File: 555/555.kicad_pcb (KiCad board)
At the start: 2 copper layers, 10 parts, among them U1 LM555xM, U2 TSOP17xx

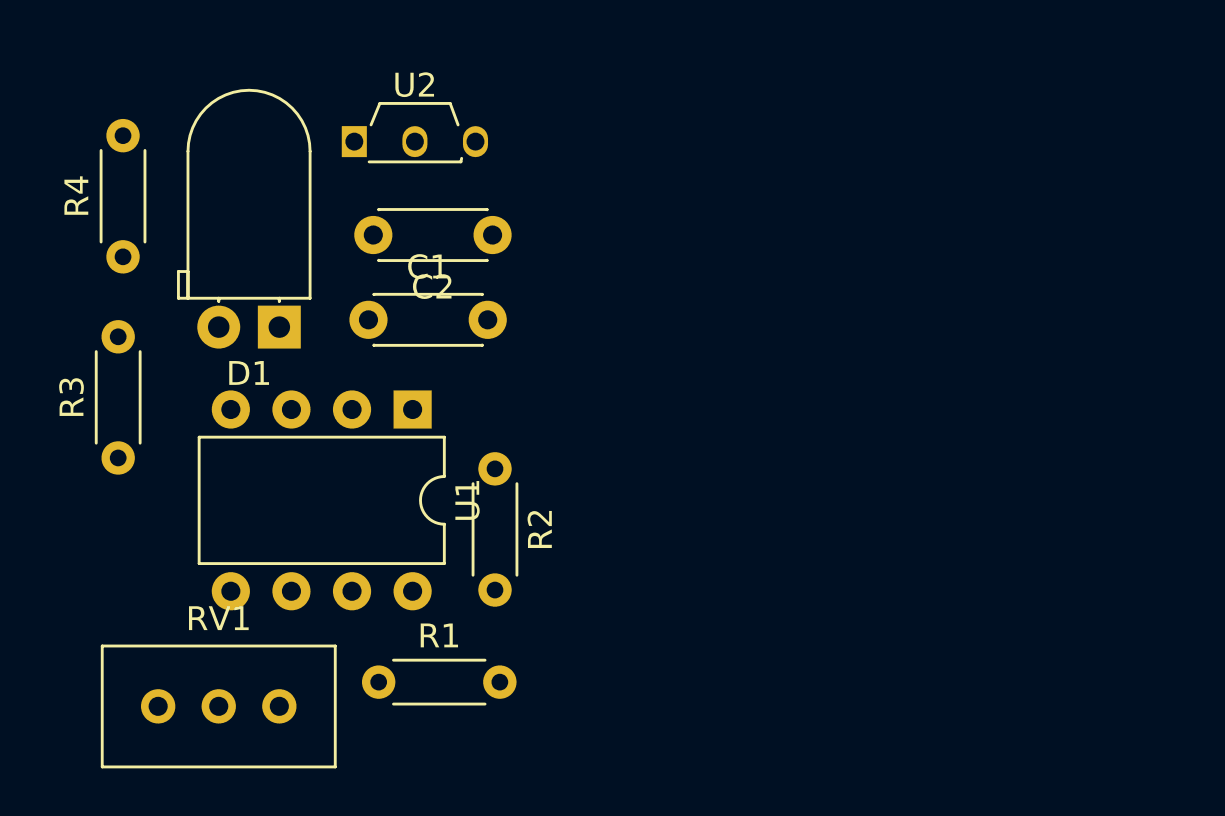
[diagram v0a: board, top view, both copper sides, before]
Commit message: 555 para imprimir
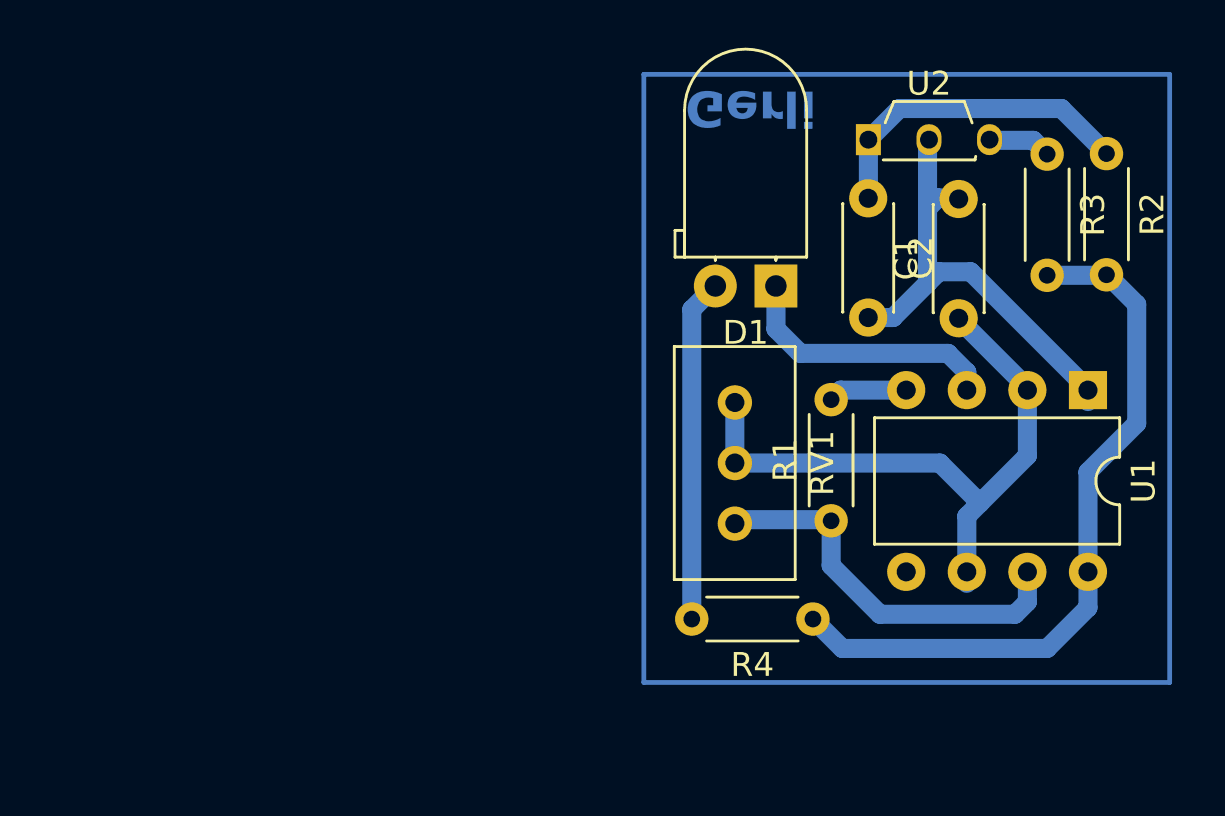
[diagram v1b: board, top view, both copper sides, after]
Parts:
- moved R3 41.0 mm to (129.5, 51.1), turned to -90 degrees
- moved R4 32.7 mm to (119.7, 70.6), turned to 180 degrees
- moved R2 28.8 mm to (132.0, 51.0)
- moved U1 28.3 mm to (131.2, 61.0)
- moved C1 24.7 mm to (125.8, 57.9), turned to 90 degrees
- moved U2 21.6 mm to (122.0, 50.5)
- moved D1 20.9 mm to (118.1, 56.6)
- moved RV1 20.6 mm to (116.4, 66.6), turned to -90 degrees
- moved R1 20.1 mm to (120.4, 66.4), turned to 90 degrees
- moved C2 15.8 mm to (122.0, 52.9), turned to -90 degrees
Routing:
- net +5V: track 0.00 -> 30.6 mm
- net Net-(U1-THR): track 0.00 -> 26.9 mm
- net GND: track 0.00 -> 20.1 mm
- net Net-(U1-DIS): track 0.00 -> 16.1 mm
- net Net-(D1-A): track 0.00 -> 14.3 mm
- net Net-(U2-GND): track 0.00 -> 13.8 mm
- net Net-(D1-K): track 0.00 -> 11.3 mm
- net Net-(U1-R): track 0.00 -> 3.31 mm
- net Sensores: track 0.00 -> 2.51 mm
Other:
- board text added: "Gerli"
